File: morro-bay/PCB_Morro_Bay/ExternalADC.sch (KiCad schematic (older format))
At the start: 89 parts, among them SW4 INPUT_RANGE_SEL_3, U10 LM2902, U11 LM2902, U12 LM2902, U26 ADS114S08BIPBSR

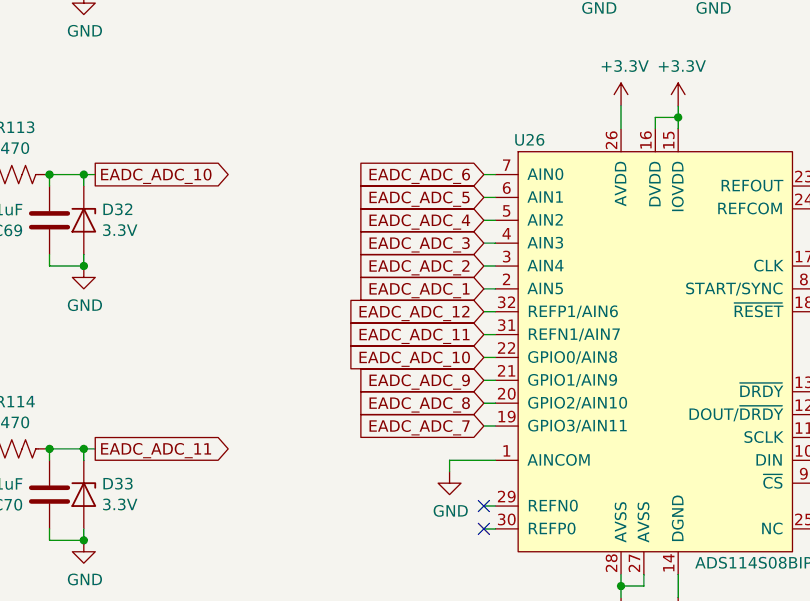
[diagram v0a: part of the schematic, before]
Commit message: More routing
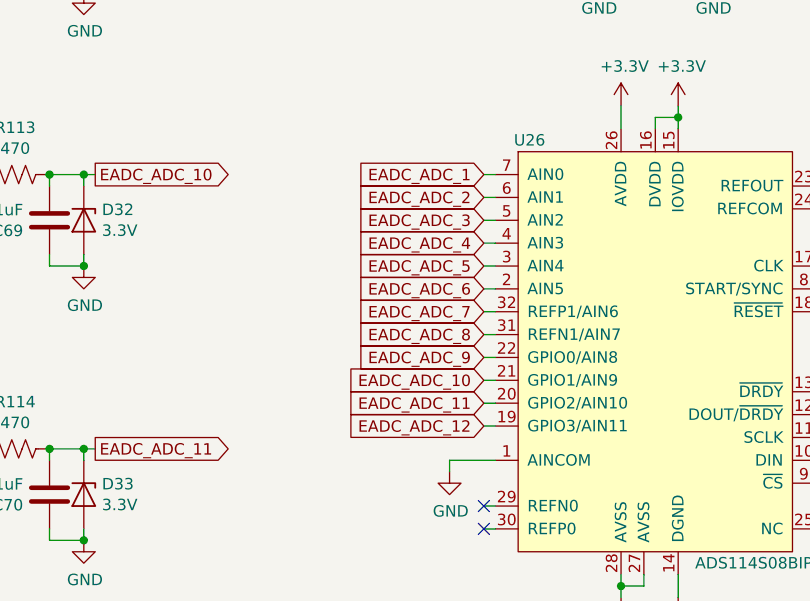
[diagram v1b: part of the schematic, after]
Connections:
- net EADC_ADC_1: now also U26.7 (AIN0); no longer U26.2 (AIN5)
- net EADC_ADC_10: now also U26.21 (GPIO1/AIN9); no longer U26.22 (GPIO0/AIN8)
- net EADC_ADC_11: now also U26.20 (GPIO2/AIN10); no longer U26.31 (REFN1/AIN7)
- net EADC_ADC_12: now also U26.19 (GPIO3/AIN11); no longer U26.32 (REFP1/AIN6)
- net EADC_ADC_2: now also U26.6 (AIN1); no longer U26.3 (AIN4)
- net EADC_ADC_3: now also U26.5 (AIN2); no longer U26.4 (AIN3)
- net EADC_ADC_4: now also U26.4 (AIN3); no longer U26.5 (AIN2)
- net EADC_ADC_5: now also U26.3 (AIN4); no longer U26.6 (AIN1)
- net EADC_ADC_6: now also U26.2 (AIN5); no longer U26.7 (AIN0)
- net EADC_ADC_7: now also U26.32 (REFP1/AIN6); no longer U26.19 (GPIO3/AIN11)
- net EADC_ADC_8: now also U26.31 (REFN1/AIN7); no longer U26.20 (GPIO2/AIN10)
- net EADC_ADC_9: now also U26.22 (GPIO0/AIN8); no longer U26.21 (GPIO1/AIN9)
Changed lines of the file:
@@
 Wire Wire Line
 	3100 1950 3050 1950
-Text GLabel 8500 2950 0    50   Input ~ 0
+Text GLabel 8500 2450 0    50   Input ~ 0
 EADC_ADC_1
 Wire Wire Line
 	8500 2450 8550 2450
-Text GLabel 8500 2850 0    50   Input ~ 0
+Text GLabel 8500 2550 0    50   Input ~ 0
 EADC_ADC_2
 Wire Wire Line
 	8500 2550 8550 2550
-Text GLabel 8500 2750 0    50   Input ~ 0
+Text GLabel 8500 2650 0    50   Input ~ 0
 EADC_ADC_3
 Wire Wire Line
 	8500 2650 8550 2650
-Text GLabel 8500 2650 0    50   Input ~ 0
+Text GLabel 8500 2750 0    50   Input ~ 0
 EADC_ADC_4
 Wire Wire Line
 	8500 2750 8550 2750
-Text GLabel 8500 2550 0    50   Input ~ 0
+Text GLabel 8500 2850 0    50   Input ~ 0
 EADC_ADC_5
 Wire Wire Line
 	8500 2850 8550 2850
-Text GLabel 8500 2450 0    50   Input ~ 0
+Text GLabel 8500 2950 0    50   Input ~ 0
 EADC_ADC_6
 Wire Wire Line
 	8500 2950 8550 2950
-Text GLabel 8500 3550 0    50   Input ~ 0
+Text GLabel 8500 3050 0    50   Input ~ 0
 EADC_ADC_7
 Wire Wire Line
 	8500 3050 8550 3050
-Text GLabel 8500 3450 0    50   Input ~ 0
+Text GLabel 8500 3150 0    50   Input ~ 0
 EADC_ADC_8
 Wire Wire Line
 	8500 3150 8550 3150
-Text GLabel 8500 3350 0    50   Input ~ 0
+Text GLabel 8500 3250 0    50   Input ~ 0
 EADC_ADC_9
 Wire Wire Line
 	8500 3250 8550 3250
-Text GLabel 8500 3250 0    50   Input ~ 0
+Text GLabel 8500 3350 0    50   Input ~ 0
 EADC_ADC_10
 Wire Wire Line
 	8500 3350 8550 3350
-Text GLabel 8500 3150 0    50   Input ~ 0
+Text GLabel 8500 3450 0    50   Input ~ 0
 EADC_ADC_11
 Wire Wire Line
 	8500 3450 8550 3450
-Text GLabel 8500 3050 0    50   Input ~ 0
+Text GLabel 8500 3550 0    50   Input ~ 0
 EADC_ADC_12
 Wire Wire Line
